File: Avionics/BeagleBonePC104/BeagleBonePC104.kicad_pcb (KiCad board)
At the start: 2 copper layers, 90.2 x 95.9 mm, 17 parts, among them U4 TJA1051T-3, U5 TMP36xS

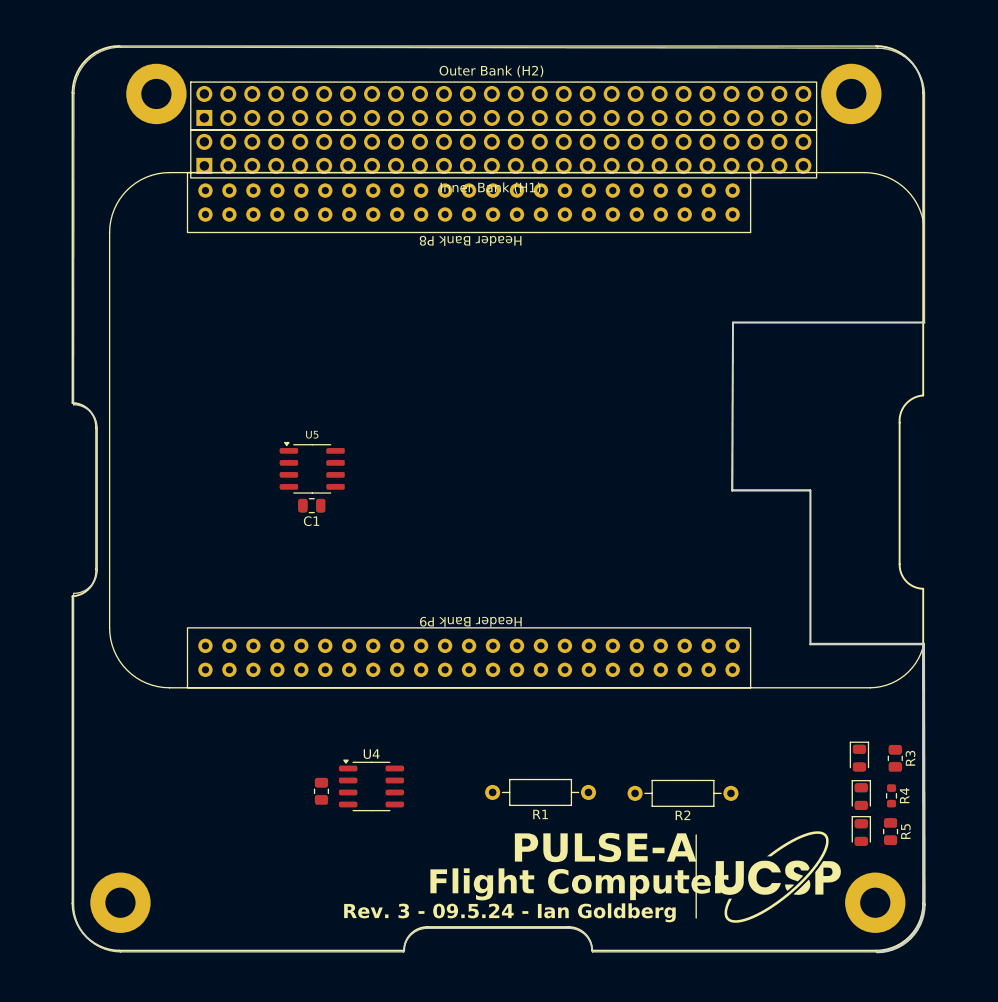
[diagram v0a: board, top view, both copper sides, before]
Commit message: Ian Golberg - Tentatively Finalized v3 of the flight computer board.
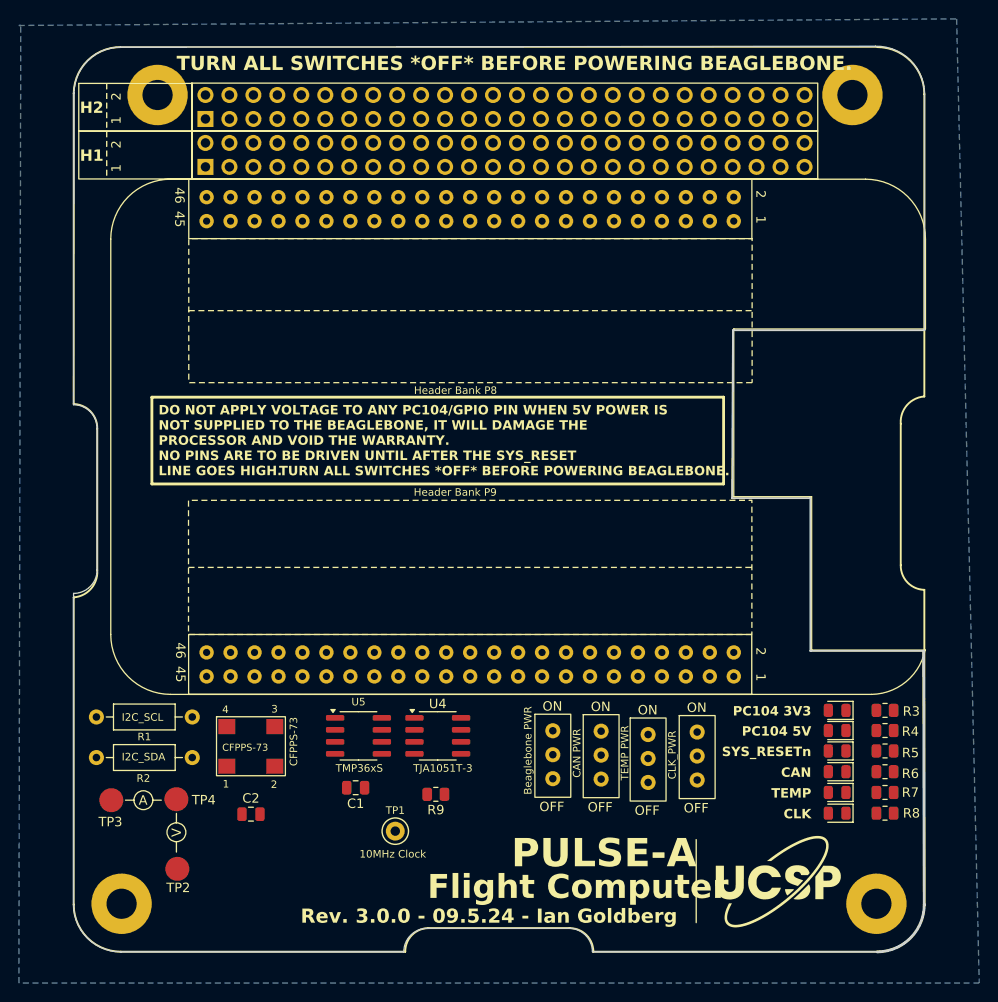
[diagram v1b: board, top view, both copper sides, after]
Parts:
- added C2: 0.1µF, Capacitor_SMD:C_0805_2012Metric, F.Cu at (98.8, 155.4)
- added D4: CAN_PWR, LED_SMD:LED_0805_2012Metric, F.Cu at (160.9, 150.9)
- added D5: TEMP_PWR, LED_SMD:LED_0805_2012Metric, F.Cu at (160.9, 153.1)
- added D6: CLK_PWR, LED_SMD:LED_0805_2012Metric, F.Cu at (160.9, 155.3)
- added R6: 15, Resistor_SMD:R_0805_2012Metric, F.Cu at (166.0, 150.9)
- added R7: 15, Resistor_SMD:R_0805_2012Metric, F.Cu at (166.0, 153.1)
- added R8: 15, Resistor_SMD:R_0805_2012Metric, F.Cu at (166.0, 155.3)
- added TP1: TestPoint, TestPoint:TestPoint_Keystone_5000-5004_Miniature, F.Cu at (114.1, 157.2)
- added TP2: TestPoint, FlightCompuer:TestPointPad, F.Cu at (90.9, 165.8)
- added TP3: TestPoint, FlightCompuer:TestPointPad, F.Cu at (83.9, 158.6)
- added TP4: TestPoint, FlightCompuer:TestPointPad, F.Cu at (95.5, 153.9)
- added U3: ~, FlightCompuer:831054046, F.Cu at (96.2, 155.3)
- added U6: ~, FlightCompuer:SPDT Through Hole Switch, F.Cu at (143.6, 154.2)
- added U7: ~, FlightCompuer:SPDT Through Hole Switch, F.Cu at (128.3, 154.1)
- added U8: ~, FlightCompuer:SPDT Through Hole Switch, F.Cu at (133.4, 154.1)
- added U9: ~, FlightCompuer:SPDT Through Hole Switch, F.Cu at (138.4, 154.5)
- R4: value 150 -> 100; footprint Resistor_SMD:R_0603_1608Metric -> Resistor_SMD:R_0805_2012Metric
- U2: footprint PCI104Connector:PCI104ConnectorComplete -> PCI104Connector:PC104ConnectorFootprint
- moved R2 57.2 mm to (92.6, 149.4)
- moved R1 42.8 mm to (92.6, 145.1)
- moved C1 30.3 mm to (109.9, 152.6)
- moved U5 28.7 mm to (110.2, 147.1)
- moved R9 12.1 mm to (118.4, 153.3), turned to 180 degrees
- moved D3 9.02 mm to (160.9, 148.7), turned to 180 degrees
- moved U4 8.84 mm to (118.6, 147.1)
- moved R5 8.57 mm to (166.0, 148.7), turned to 0 degrees
- moved D2 7.46 mm to (160.9, 146.5), turned to 180 degrees
- moved R4 6.96 mm to (166.0, 146.5), turned to 0 degrees
- moved D1 5.59 mm to (160.9, 144.4), turned to 180 degrees
- moved R3 5.20 mm to (166.0, 144.4), turned to 0 degrees
- moved U1 0.71 mm to (170.3, 88.1)
- moved G*** 0.49 mm to (154.5, 162.6)
- moved U2 0.16 mm to (80.0, 170.0)
- renumbered R6 to R9
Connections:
- C1 pad 1: /3V3 -> Net-(D5-A)
- R1 pad 1: /5V -> Net-(R1-Pad1)
- R2 pad 1: /5V -> Net-(R1-Pad1)
- U1 pad 23: /GPIO1_17 -> /FC_TEMP
- U1 pad 5: /5V -> Net-(R1-Pad1)
- U1 pad 6: /5V -> Net-(R1-Pad1)
- U1 pad 83: unconnected-(U1-UART5_TXD-Pad83) -> /UART_TX
- U1 pad 84: unconnected-(U1-UART5_RXD-Pad84) -> /UART_RX
- U2 pad 103: unconnected-(U2-Pad103) -> /10MHz_CLK
- U2 pad 19: unconnected-(U2-UART_1_TX-Pad19) -> /UART_TX
- U2 pad 20: unconnected-(U2-UART_1_RX-Pad20) -> /UART_RX
- U2 pad 36: /GPIO2_6 -> unconnected-(U2-Pad36)
- U2 pad 53: /FC_TEMP -> unconnected-(U2-TEMP_1-Pad53)
- U2 pad 70: unconnected-(U2-Pad70) -> /GPIO2_6
- U2 pad 80: unconnected-(U2-Pad80) -> /3V3
- U2 pad 96: /GPIO1_17 -> /FC_TEMP
- U4 pad 3: /3V3 -> Net-(D4-A)
- U4 pad 5: /3V3 -> Net-(D4-A)
- U5 pad 5: /3V3 -> Net-(D5-A)
- U5 pad 8: /3V3 -> Net-(D5-A)
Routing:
- net /GPIO1_15: track 0.00 -> 0.82 mm
- added copper zone on In2.Cu, net /3V3
- added copper zone on B.Cu, net GND
- added copper zone on In1.Cu, net GND
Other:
- board size 90.2 x 95.9 mm -> 90.2 x 96 mm
- copper layers 2 -> 4
- board text added: "10MHz Clock"
- board text added: "A"
- board text added: "Beaglebone PWR"
- board text added: "CAN"
- board text added: "CAN PWR"
- board text added: "CFPPS-73"
- board text added: "CLK"
- board text added: "CLK_PWR"
- board text added: "DO NOT APPLY VOLTAGE TO ANY PC104/GPIO PIN WHEN 5V POWER IS NOT SUPPLIED TO THE BEAGLEBONE, IT WILL DAMAGE THE PROCESSOR AND VOID THE WARRANTY. NO PINS ARE TO BE DRIVEN UNTIL AFTER THE SYS_RESET LINE GOES HIGH."
- board text added: "I2C_SCL"
- board text added: "I2C_SDA"
- board text added: "PC104 3V3"
- board text added: "PC104 5V"
- board text added: "Rev. 3.0.0 - 09.5.24 - Ian Goldberg"
- board text added: "SYS_RESETn"
- board text added: "TEMP"
- board text added: "TEMP PWR"
- board text added: "TJA1051T-3"
- board text added: "TMP36xS"
- board text added: "TURN ALL SWITCHES *OFF* BEFORE POWERING BEAGLEBONE."
- board text added: "V"
- board text added: "{dblquote}Do, or do not. There is no try.{dblquote} -Yoda"
- board text removed: "Rev. 3 - 09.5.24 - Ian Goldberg"
